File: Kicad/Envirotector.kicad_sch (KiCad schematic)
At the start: 3 parts, among them J1 OLED Display, U1 XIAO-RP2040-DIP, U2 DHT11

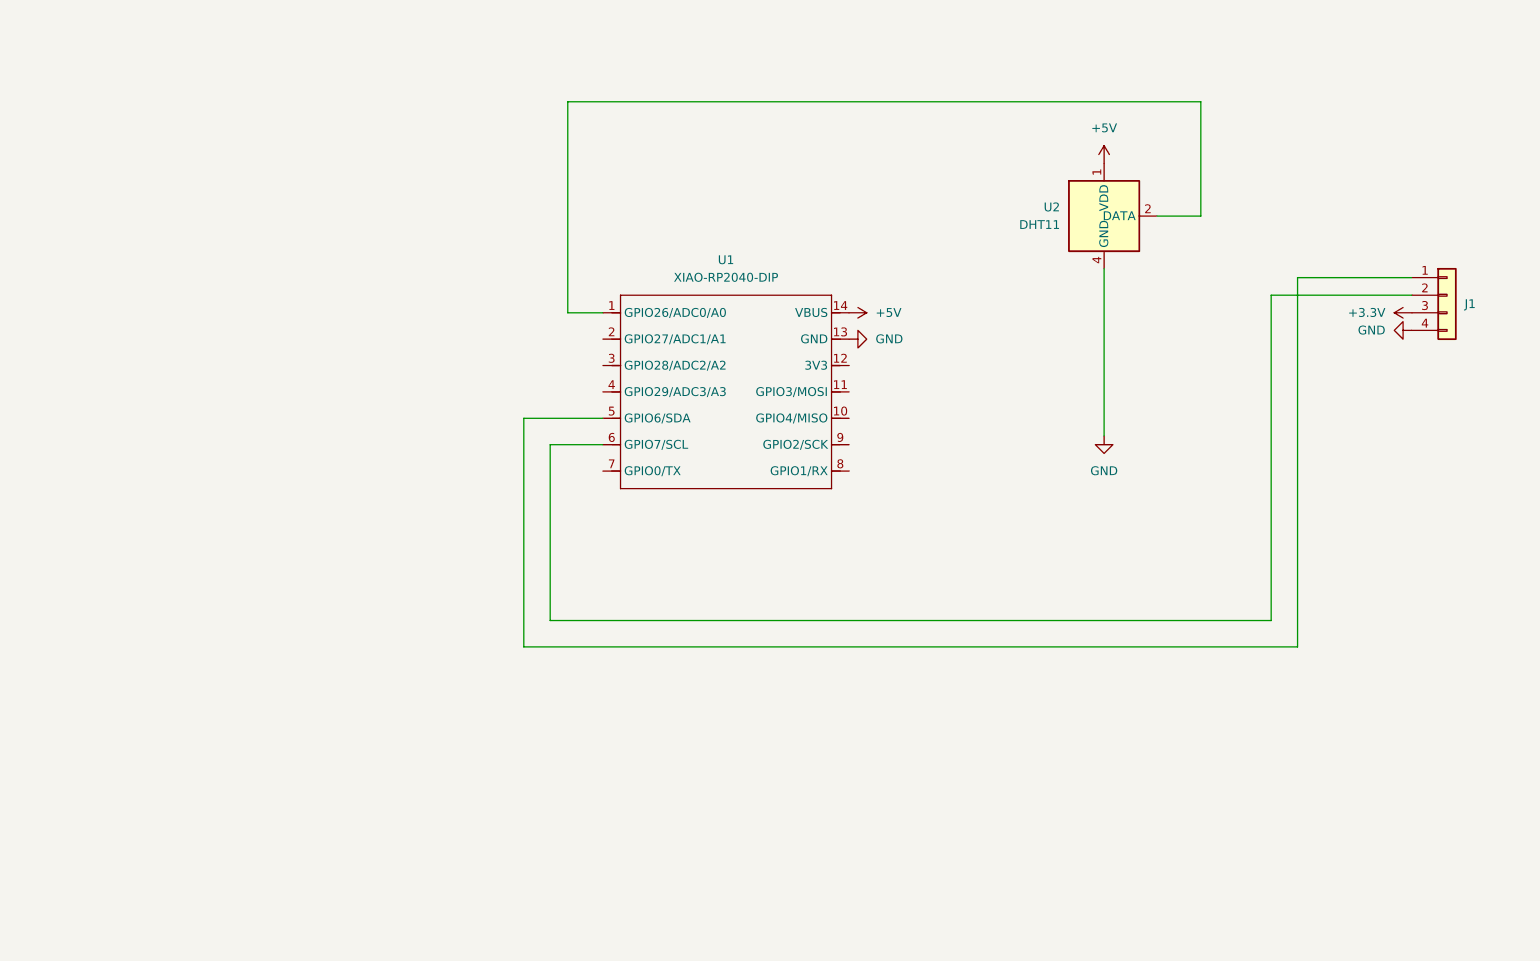
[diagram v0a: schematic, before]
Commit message: Upload
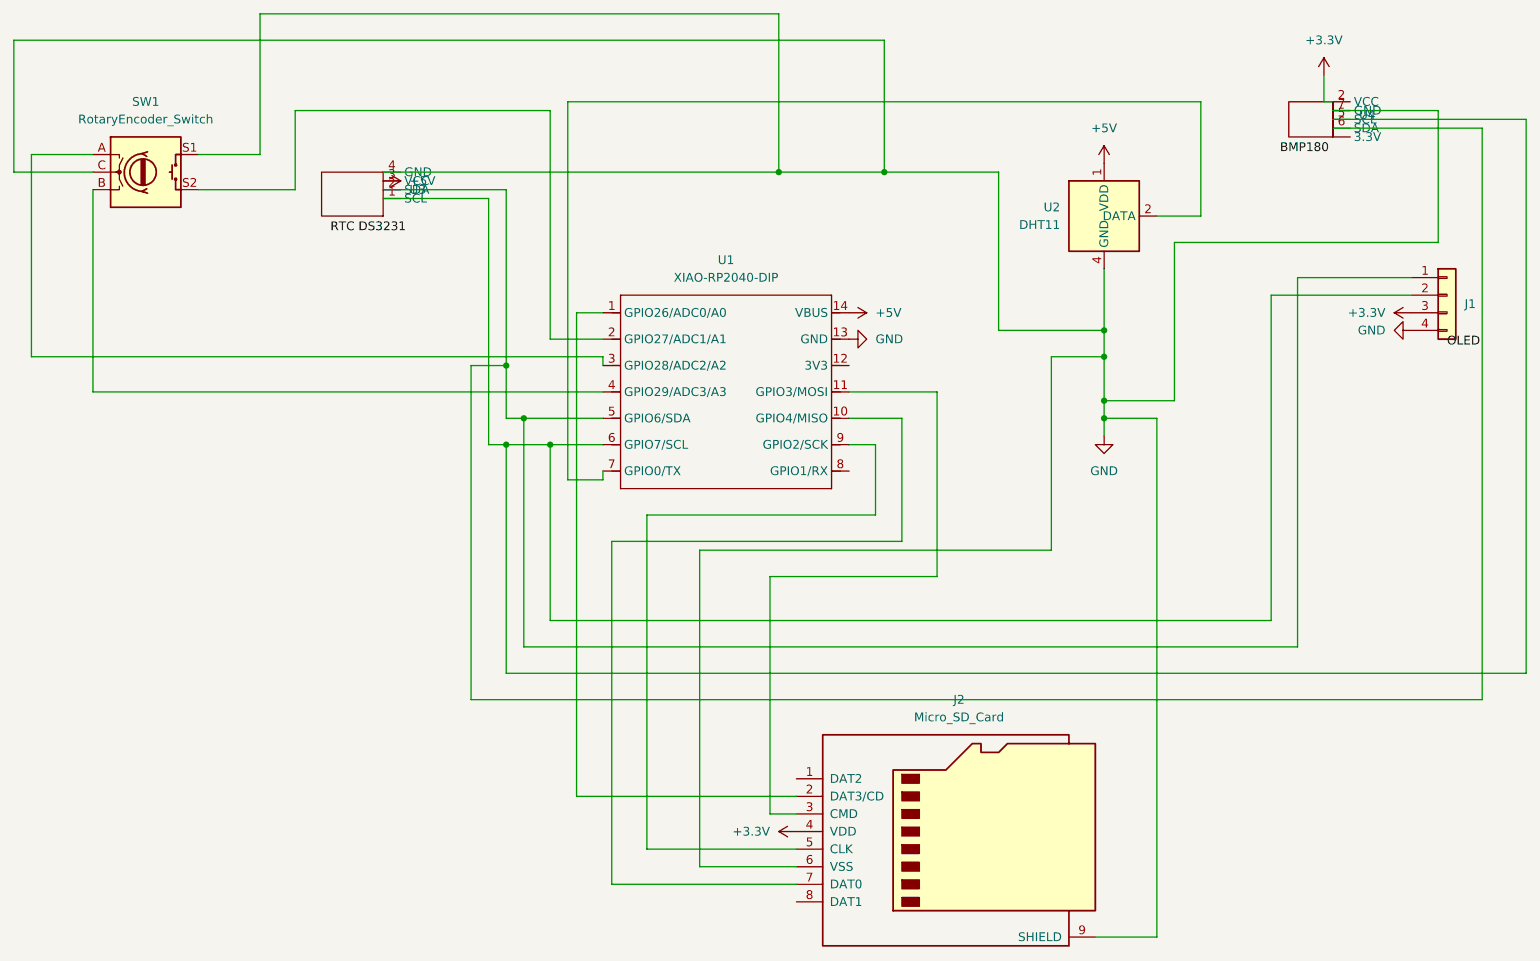
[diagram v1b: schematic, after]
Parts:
- added J2: Micro_SD_Card, Connector_Card:microSD_HC_Hirose_DM3AT-SF-PEJM5, symbol Connector:Micro_SD_Card
- added SW1: RotaryEncoder_Switch, Rotary_Encoder:RotaryEncoder_Alps_EC11E-Switch_Vertical_H20mm, symbol Device:RotaryEncoder_Switch
- added U3: ~, LARGE:RTC_DS3231, symbol RTC:RTC_DS3231
- added U4: ~, SPARK:BMP180, symbol BMP:BMP180
- U1: footprint OPL:XIAO-RP2040-DIP -> Module:MOUDLE14P-XIAO-DIP-SMD
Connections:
- net +3.3V: now also J2.4 (VDD), U4.2 (VCC)
- net +5V: now also U3.3 (VCC)
- net GND: now also J2.6 (VSS), J2.9 (SHIELD), SW1.C, SW1.S1, U3.4 (GND), U4.7 (GND)
- net at J1.1 (Pin_1), U1.5 (GPIO6/SDA): now also U3.2 (SDA), U4.6 (SDA)
- net at J1.2 (Pin_2), U1.6 (GPIO7/SCL): now also U3.1 (SCL), U4.5 (SCL)
- net at U1.1 (GPIO26/ADC0/A0): now also J2.2 (DAT3/CD); no longer U2.2 (DATA)
- net at U1.10 (GPIO4/MISO): now also J2.7 (DAT0)
- net at U1.11 (GPIO3/MOSI): now also J2.3 (CMD)
- net at U1.2 (GPIO27/ADC1/A1): now also SW1.S2
- net at U1.3 (GPIO28/ADC2/A2): now also SW1.A
- net at U1.4 (GPIO29/ADC3/A3): now also SW1.B
- net at U1.7 (GPIO0/TX): now also U2.2 (DATA)
- net at U1.9 (GPIO2/SCK): now also J2.5 (CLK)
